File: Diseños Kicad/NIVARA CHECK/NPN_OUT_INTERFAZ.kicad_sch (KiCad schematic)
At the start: 6 parts, among them K1 G2RL-1, K2 G2RL-1, Q1 NCV8402xST, Q2 NCV8402xST

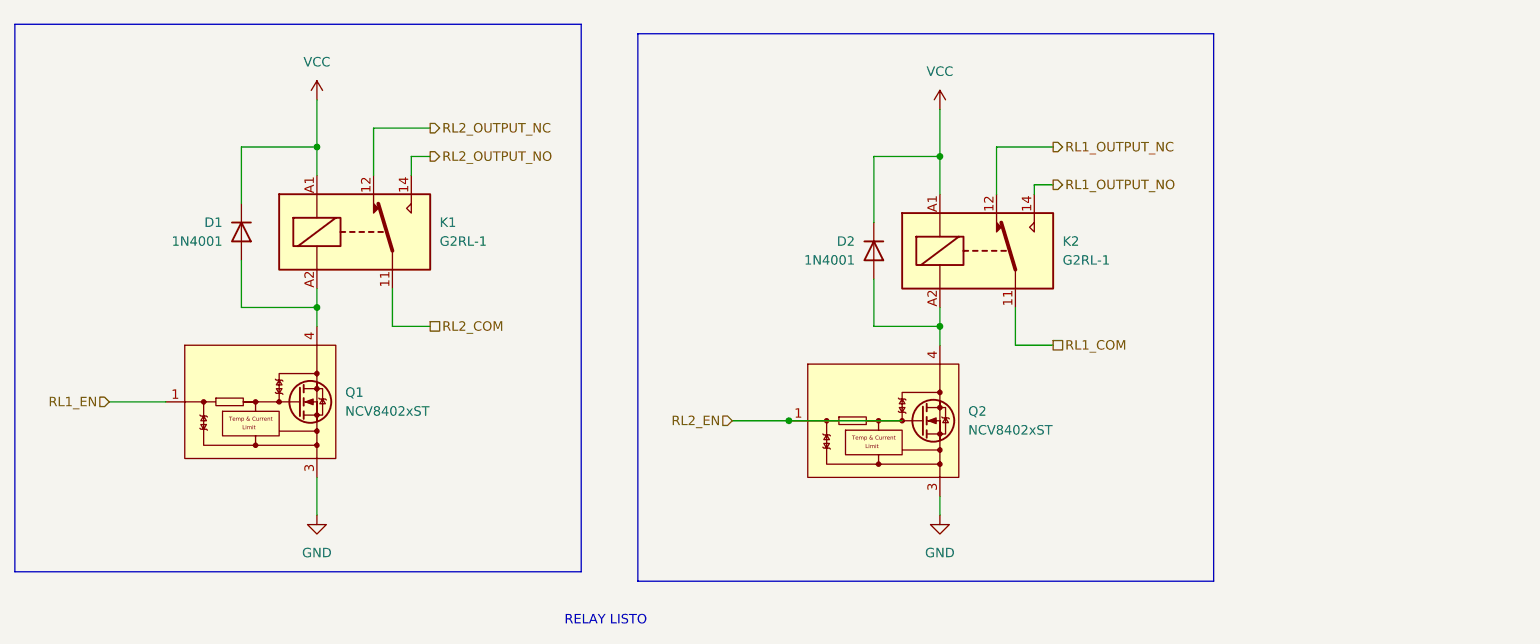
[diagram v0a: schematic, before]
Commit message: ACTUALIZACION HECHA
PCB SUPUESTA
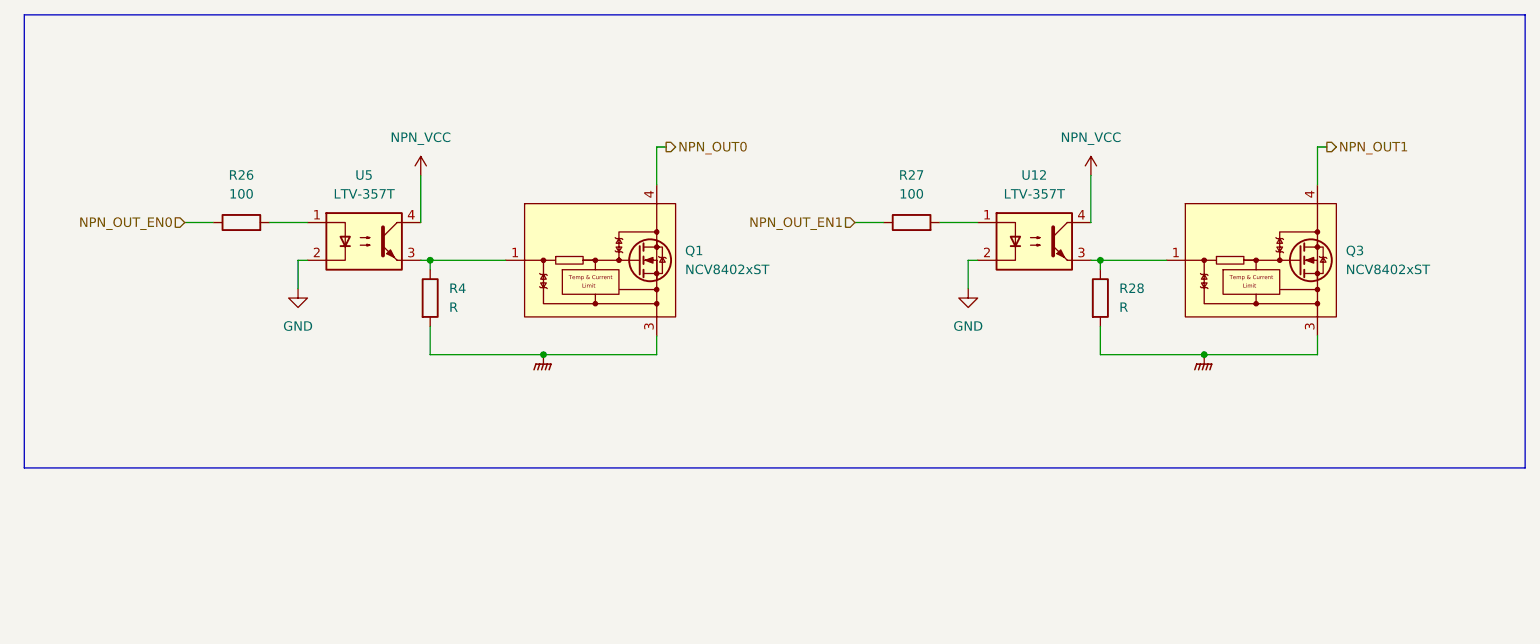
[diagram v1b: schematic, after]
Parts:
- removed D1, D2: 1N4001, Diode_SMD:D_SMA, symbol Diode:1N4001
- removed K1, K2: G2RL-1, Relay_THT:Relay_SPDT_Omron_G2RL-1, symbol Relay:G2RL-1
- removed Q2: NCV8402xST, Package_TO_SOT_SMD:SOT-223, symbol Driver_FET:NCV8402xST
- added Q3: NCV8402xST, Package_TO_SOT_SMD:SOT-223, symbol Driver_FET:NCV8402xST
- added R26, R27: 100, symbol Device:R
- added R28, R4: R, symbol Device:R
- added U12, U5: LTV-357T, Package_SO:SO-4_4.4x3.6mm_P2.54mm, symbol Isolator:LTV-357T
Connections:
- net GND: now also U12.2, U5.2; no longer Q1.3 (S)
- net NPN_OUT0: now reaches Q1.2 (D), Q1.4 (D)
- net RL1_EN: no longer names the net of Q1.1 (G)
- net RL1_EN: now also R4.1, U5.3
- new net: Q3.1 (G), R28.1, U12.3
- new net: R26.2, U5.1
- new net: R27.2, U12.1
- new net NPNOUT_GND: Q1.3 (S), Q3.3 (S), R28.2, R4.2
- new net NPN_OUT1: Q3.2 (D), Q3.4 (D)
- new net NPN_OUT_EN0: R26.1
- new net NPN_OUT_EN1: R27.1
- new net NPN_VCC: U12.4, U5.4
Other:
- note removed: "RELAY LISTO"
- moved on the sheet: Q1
